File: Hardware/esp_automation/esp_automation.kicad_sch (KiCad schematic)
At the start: 12 parts, among them J1 UART, SW1 RESET, SW2 BOOT, U1 ESP32-WROOM-32D

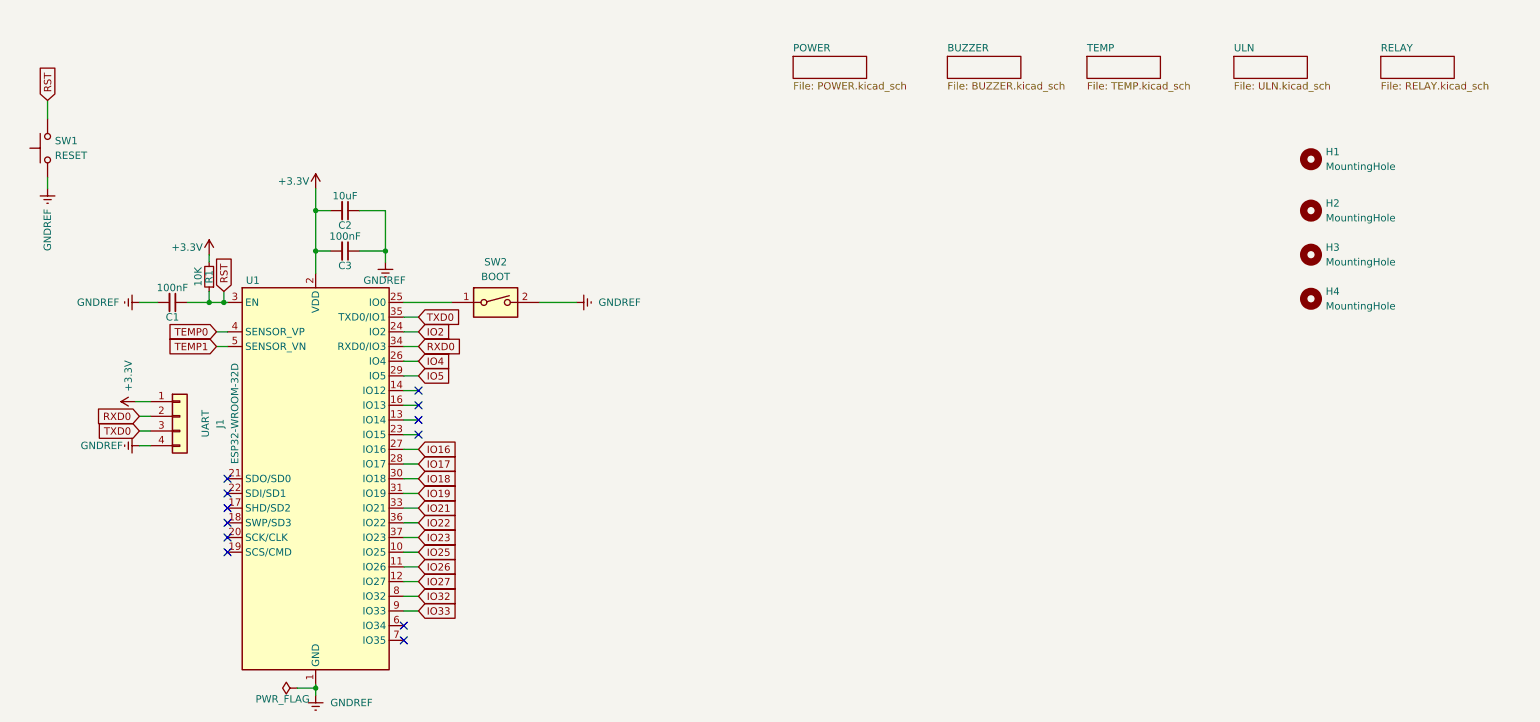
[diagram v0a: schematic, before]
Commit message: add software
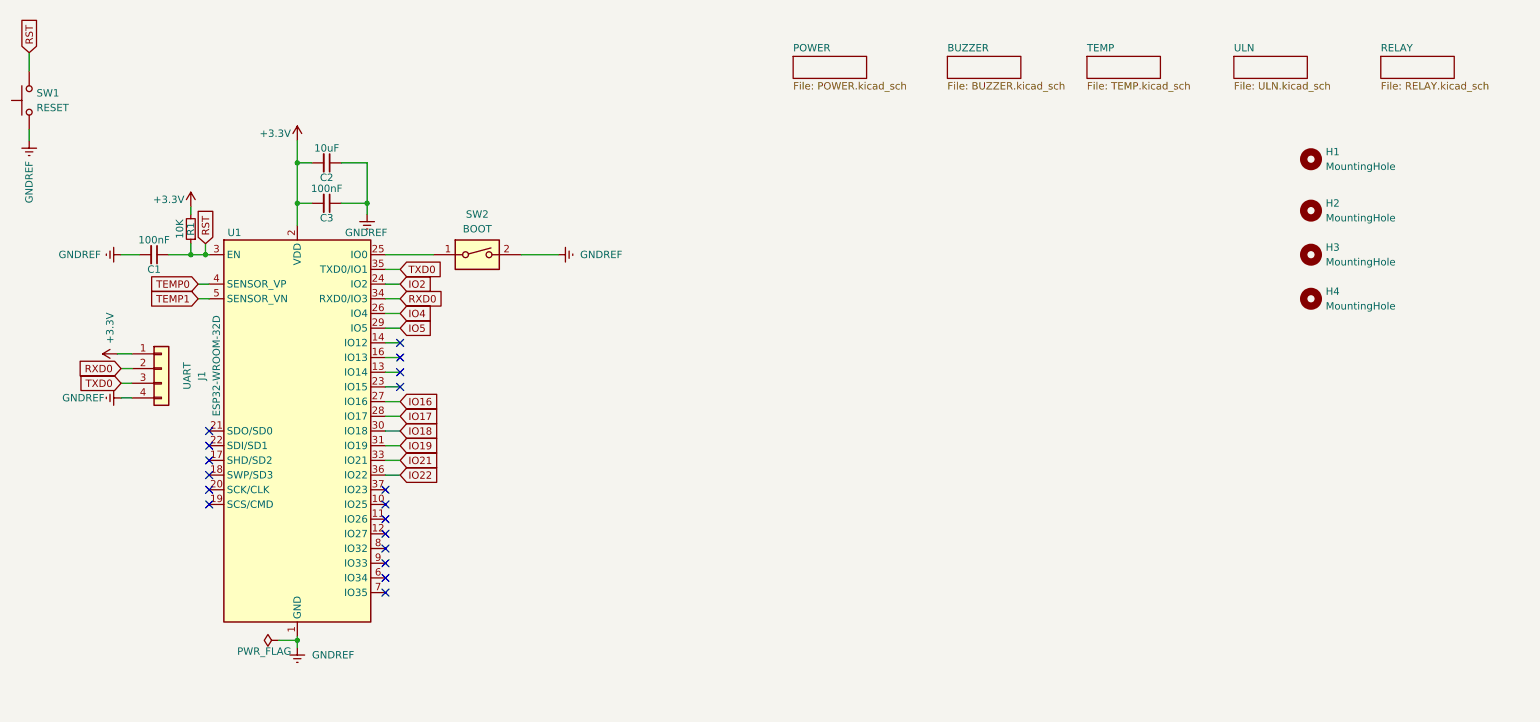
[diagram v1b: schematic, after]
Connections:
- net IO23: no longer names the net of U1.37 (IO23)
- net IO25: no longer names the net of U1.10 (IO25)
- net IO26: no longer names the net of U1.11 (IO26)
- net IO27: no longer names the net of U1.12 (IO27)
- net IO32: no longer names the net of U1.8 (IO32)
- net IO33: no longer names the net of U1.9 (IO33)
- no-connect marks 12 -> 18
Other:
- moved on the sheet: C1, C2, C3, J1, R1, SW1, SW2, U1
